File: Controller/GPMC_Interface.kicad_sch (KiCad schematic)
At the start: 37 parts, among them J61 TC2050, SW1 SW_DIP_x04, SW3 SW_Push, SW4 SW_Push, U11 AM6252ASGFHIAMCRQ1

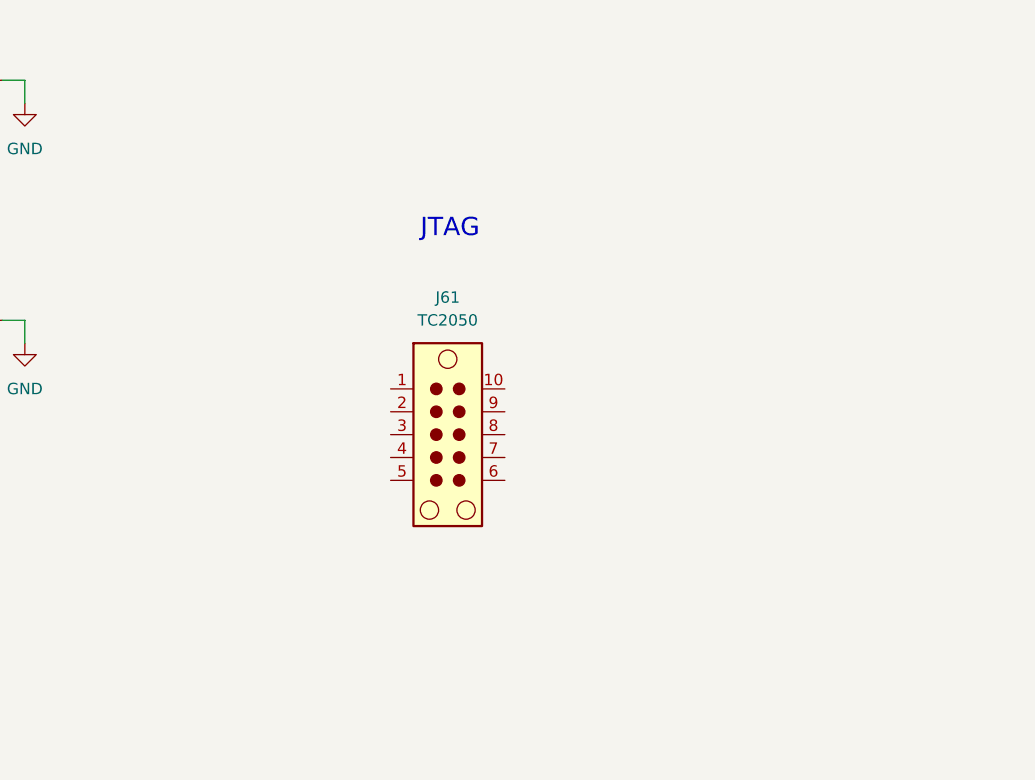
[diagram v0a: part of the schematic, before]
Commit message: JTAG
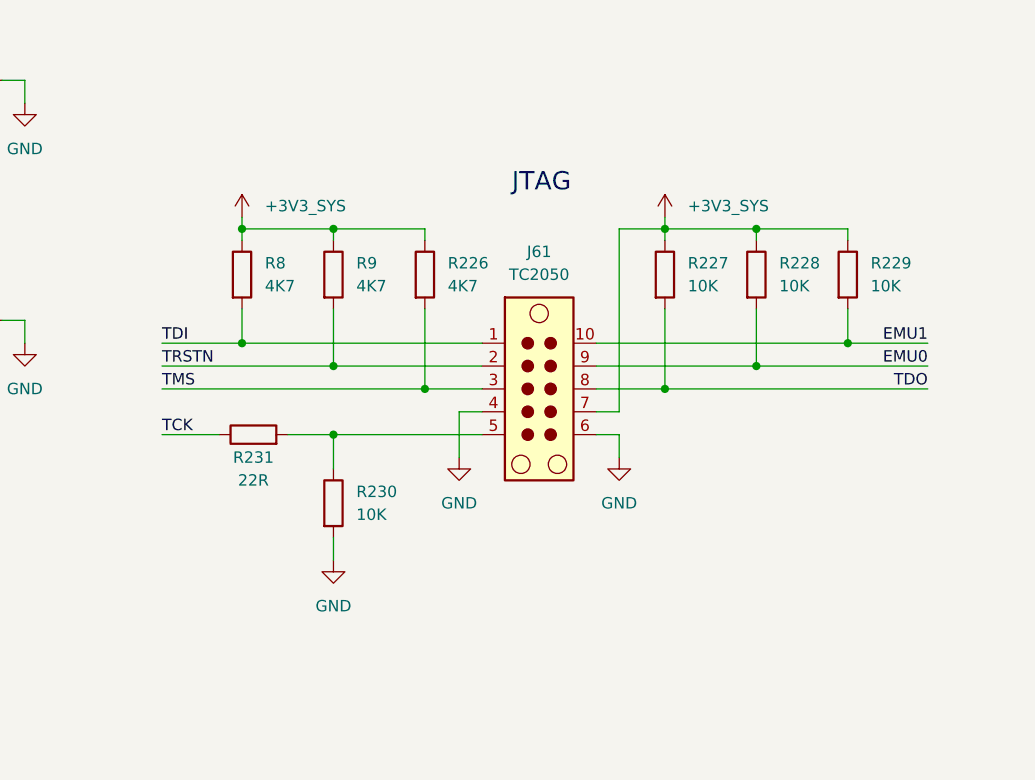
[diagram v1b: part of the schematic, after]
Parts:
- added R226, R8, R9: 4K7, Resistor_SMD:R_0603_1608Metric, symbol Device:R
- added R227, R228, R229, R230: 10K, Resistor_SMD:R_0603_1608Metric, symbol Device:R
- added R231: 22R, Resistor_SMD:R_0402_1005Metric, symbol Device:R
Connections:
- net +3V3_SYS: now also J61.7, R226.1, R227.1, R228.1, R229.1, R8.1, R9.1
- net EMU0: now also J61.9, R228.2
- net EMU1: now also J61.10, R229.2
- net GND: now also J61.4, J61.6, R230.2
- net TCK: now also R231.1
- net TDI: now also J61.1, R8.2
- net TDO: now also J61.8, R227.2
- net TMS: now also J61.3, R226.2
- net TRSTN: now also J61.2, R9.2
- net at J61.5: now also R230.1, R231.2
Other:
- moved on the sheet: J61
